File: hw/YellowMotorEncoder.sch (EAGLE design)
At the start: 20 parts, among them P1 M1

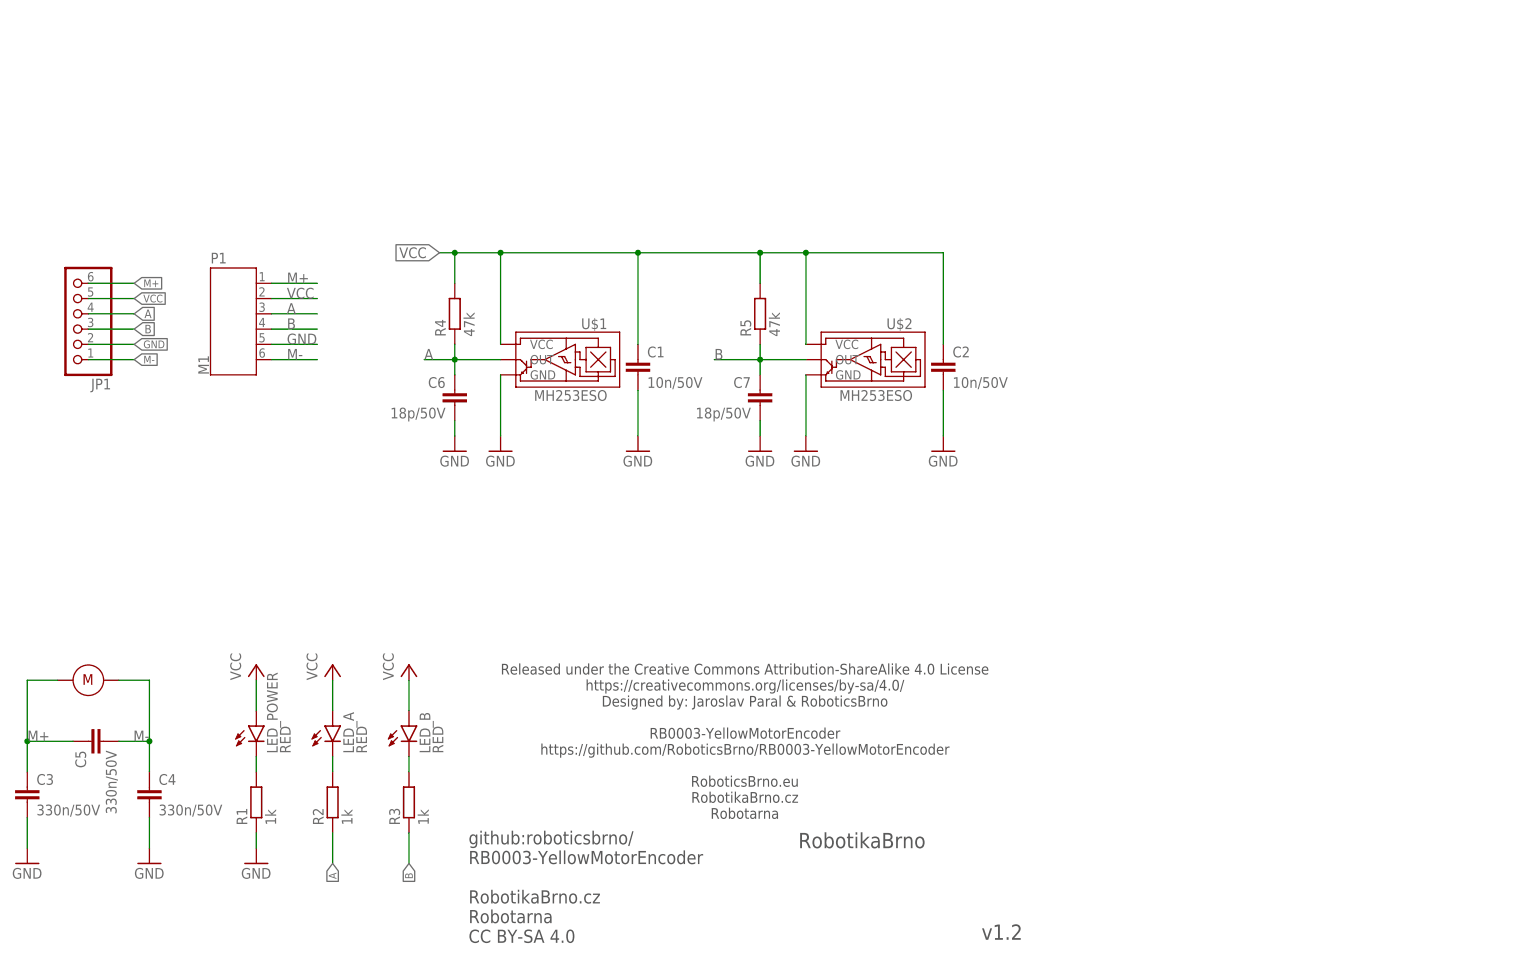
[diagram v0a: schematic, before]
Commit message: FourProbes
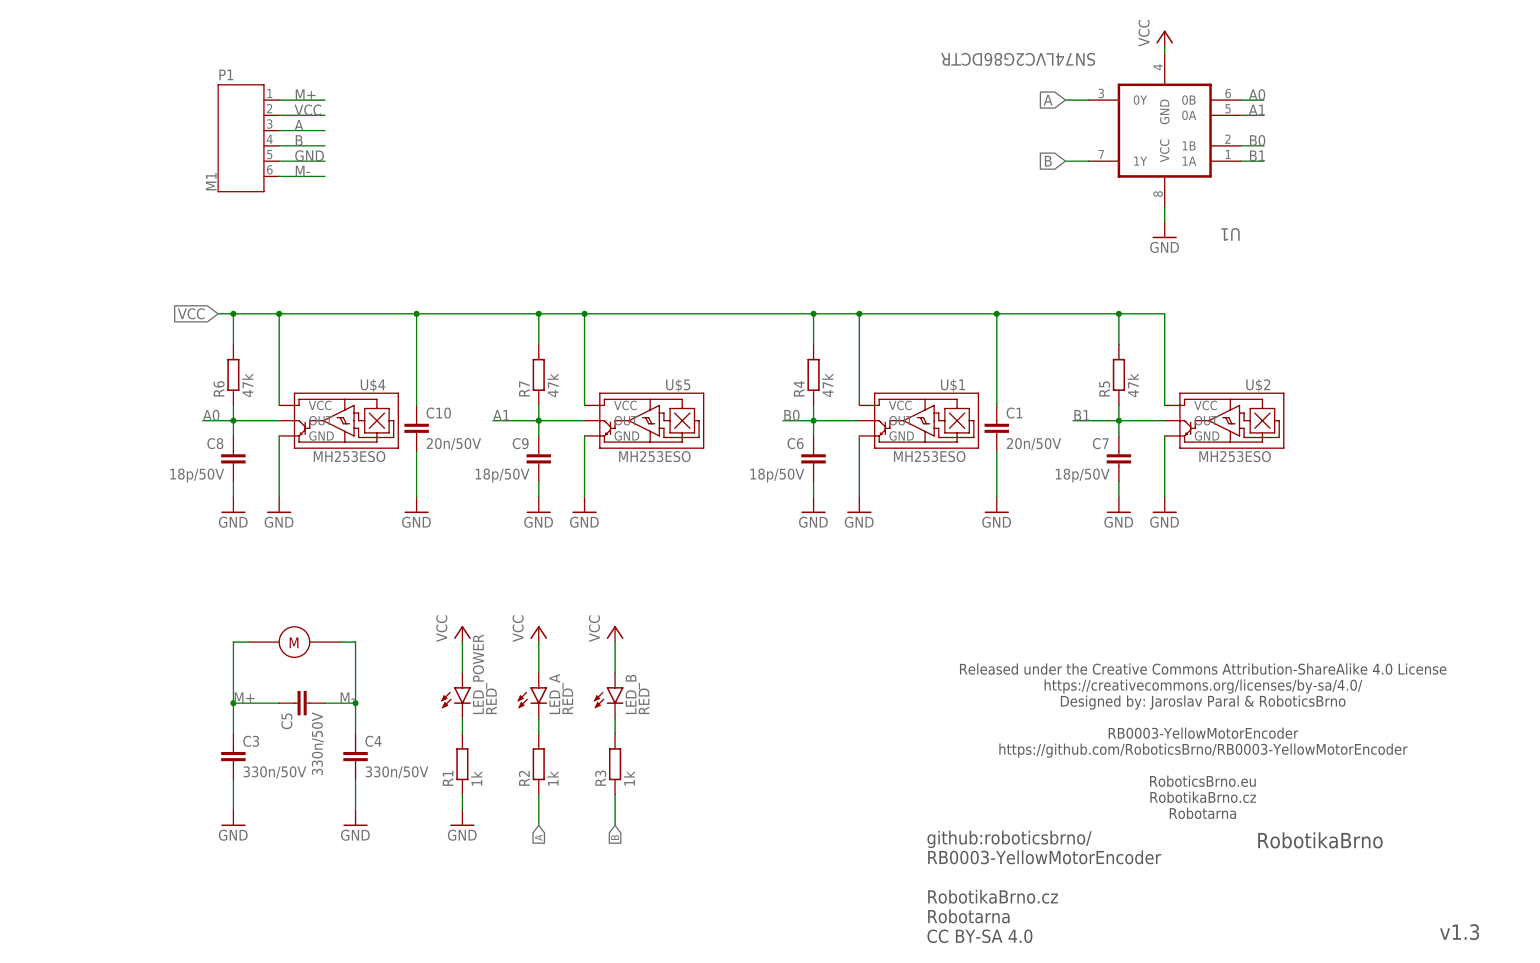
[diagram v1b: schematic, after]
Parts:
- removed C2: 10n/50V, rcl:C-EUC0402
- removed JP1: (no value), pinhead:PINHD-1X6
- removed U$3: YELLOW_MOTOR, motor:YELLOW_MOTOR
- added C10: 20n/50V, rcl:C-EUC0402
- added C8, C9: 18p/50V, rcl:C-EUC0402
- added M1: MOTOR, motor:MOTOR
- added R6, R7: 47k, rcl:R-EU_R0402
- added U$4, U$5: MH253ESO, hall_sensor:MH253ESO
- added U1: SN74LVC2G86DCTR, SN74LVC2G86DCTR:SN74LVC2G86DCTR
- C1: value 10n/50V -> 20n/50V
- R1, R2, R3, R4, R5: device rcl:R-EU_R0603 -> rcl:R-EU_R0402
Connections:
- new net A0: C8.1, R6.1, U$4.OUT, U1.0B
- new net A1: C9.1, R7.1, U$5.OUT, U1.0A
- new net B0: C6.1, R4.1, U$1.OUT, U1.1B
- new net B1: C7.1, R5.1, U$2.OUT, U1.1A
- net A: now also U1.0Y; no longer C6.1, JP1.4, R4.1, U$1.OUT
- net B: now also U1.1Y; no longer C7.1, JP1.3, R5.1, U$2.OUT
- net GND: now also C10.2, C8.2, C9.2, U$4.GND, U$5.GND, U1.VCC; no longer C2.2, JP1.2
- net M+: now also M1.P$1; no longer JP1.6, U$3.P$2
- net M-: now also M1.P$2; no longer JP1.1, U$3.P$1
- net VCC: now also C10.1, R6.2, R7.2, U$4.VCC, U$5.VCC, U1.GND; no longer C2.1, JP1.5
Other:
- note added: "v1.3"
- note removed: "v1.2"
- moved on the sheet: C1, C3, C4, C5, C6, C7, LED_A, LED_B, LED_POWER, P1, R1, R2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
